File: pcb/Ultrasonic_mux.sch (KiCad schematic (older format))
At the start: 71 parts, among them J0 DB9_Male, J2 DB9_Male, J3 DB9_Male, J4 DB9_Male, J5 DB9_Male, J8 DB9_Male, Q0 MMBT3904, Q2 MMBT3904, Q3 MMBT3904, Q4 MMBT3904, Q5 MMBT3904, Q8 MMBT3904, U1 FeatherM0

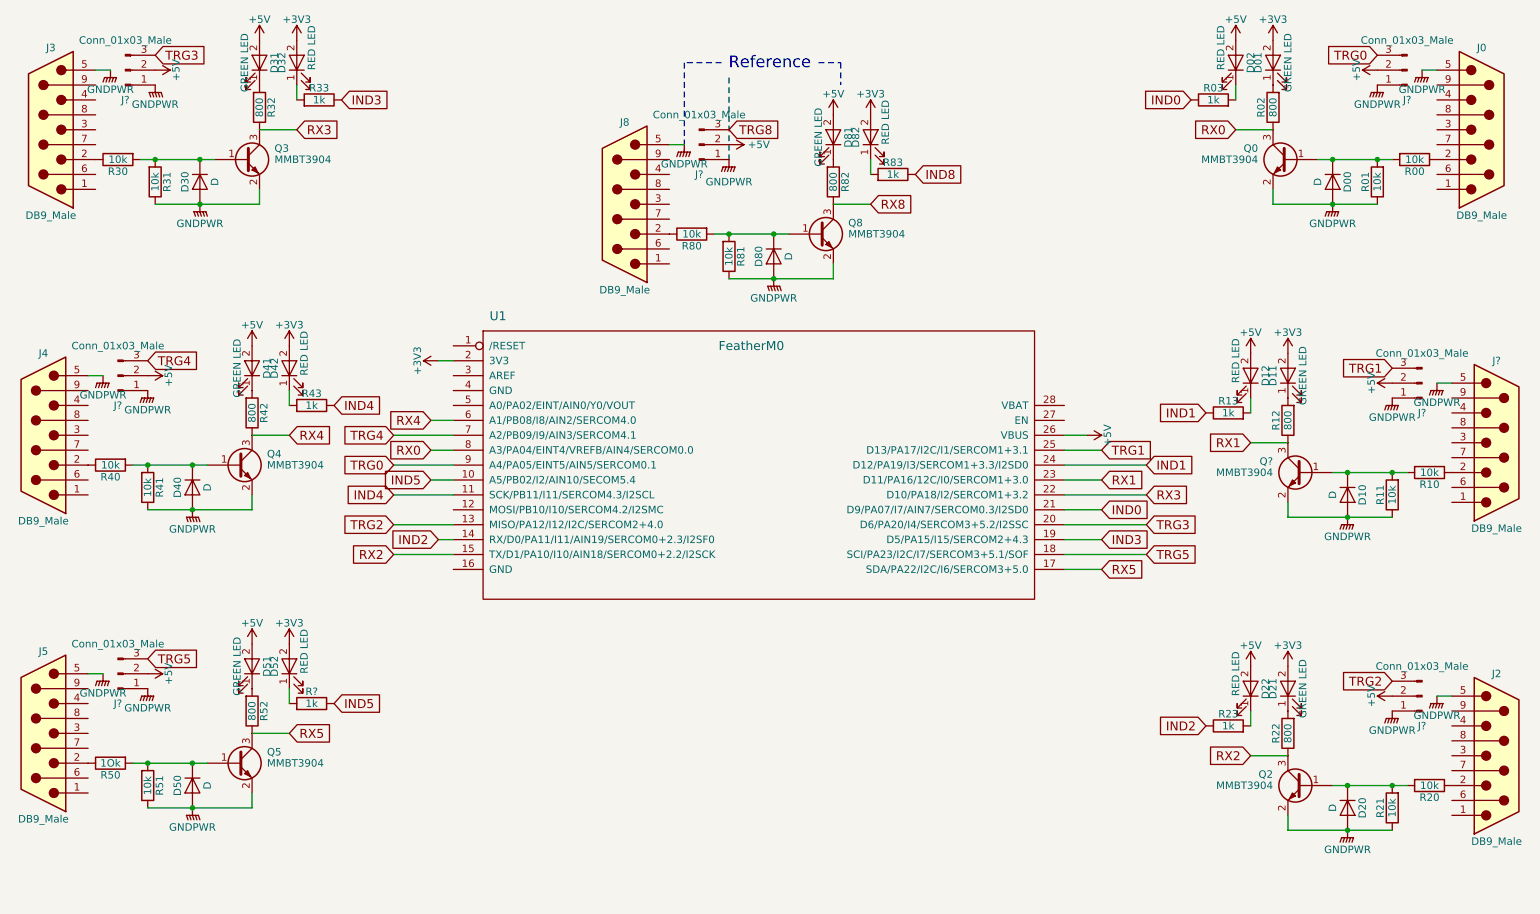
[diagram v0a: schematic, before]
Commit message: Finished schematic
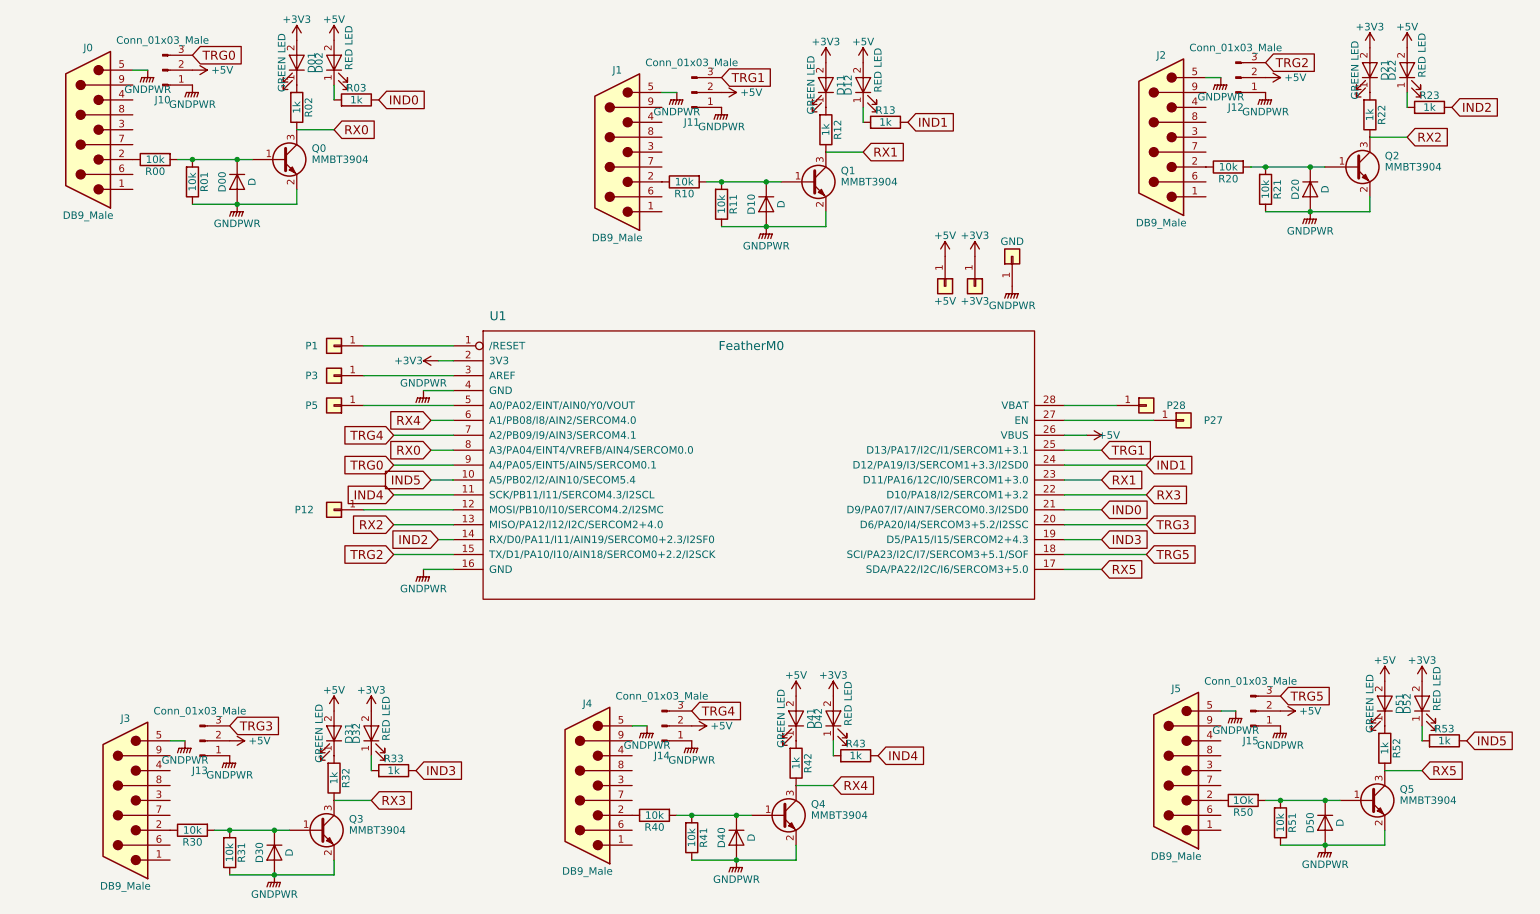
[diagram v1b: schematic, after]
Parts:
- removed D80: D, symbol D
- removed D81: GREEN LED, symbol LED
- removed D82: RED LED, symbol LED
- removed J8: DB9_Male, symbol DB9_Male
- removed J?: Conn_01x03_Male, symbol Conn_01x03_Male
- removed Q8: MMBT3904, TO_SOT_Packages_SMD:SOT-23, symbol MMBT3904
- removed R80, R81: 10k, symbol R
- removed R82: 800, symbol R
- removed R83: 1k, symbol R
- added +3V3, +5V, GND, P1, P12, P27, P28, P3, P5: (no value), symbol Conn_01x01
- R02, R12, R22, R32, R42, R52: value 800 -> 1k
- gave numbers to parts that had none: 9
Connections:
- net +3V3: now also +3V3.1 (Pin_1)
- net +5V: now also +5V.1 (Pin_1)
- net GNDPWR: now also U1.16 (GND), U1.4 (GND), GND.1 (Pin_1)
- net RX2: now also U1.13 (MISO/PA12/I12/I2C/SERCOM2+4.0); no longer U1.15 (TX/D1/PA10/I10/AIN18/SERCOM0+2.2/I2SCK)
- net TRG2: now also U1.15 (TX/D1/PA10/I10/AIN18/SERCOM0+2.2/I2SCK); no longer U1.13 (MISO/PA12/I12/I2C/SERCOM2+4.0)
- net at U1.1 (/RESET): now also P1.1 (Pin_1)
- net at U1.12 (MOSI/PB10/I10/SERCOM4.2/I2SMC): now also P12.1 (Pin_1)
- net at U1.27 (EN): now also P27.1 (Pin_1)
- net at U1.28 (VBAT): now also P28.1 (Pin_1)
- net at U1.3 (AREF): now also P3.1 (Pin_1)
- net at U1.5 (A0/PA02/EINT/AIN0/Y0/VOUT): now also P5.1 (Pin_1)
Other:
- note removed: "Reference"
- moved on the sheet: D00, D01, D02, D10, D11, D12, D20, D21, D22, D30, D31, D32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
